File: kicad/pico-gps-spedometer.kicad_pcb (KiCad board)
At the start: 2 copper layers, 88.1 x 75.5 mm, 28 parts, among them J1 Akkumulátor be, J2 TP4056-18650-Charger, J3 uBlox NEO GPS (6M/8M), Q1 PN2222A, Q2 BC212, U1 RP2040-ZERO, U2 DS18B20, U3 LM7805_TO220, U4 TFT_320x240

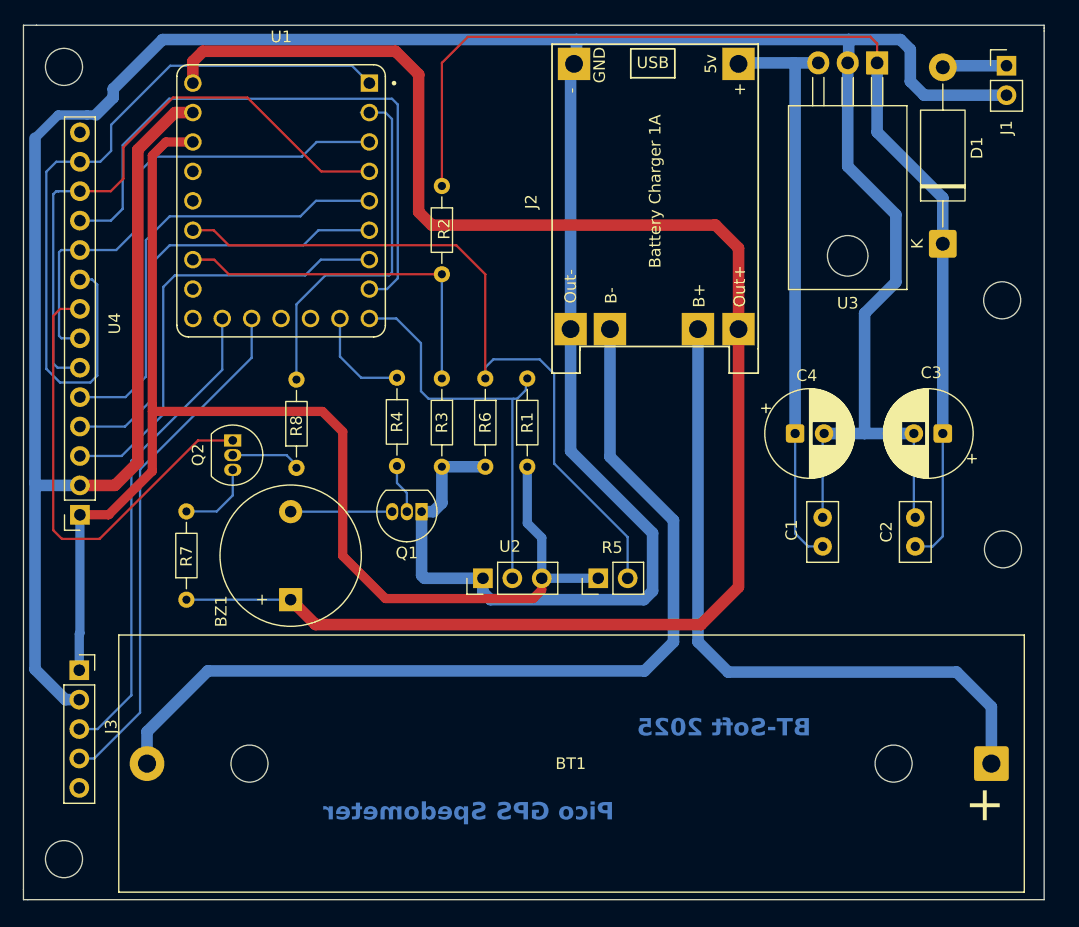
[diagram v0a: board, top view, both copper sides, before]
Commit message: Refactor code structure for improved readability and maintainability
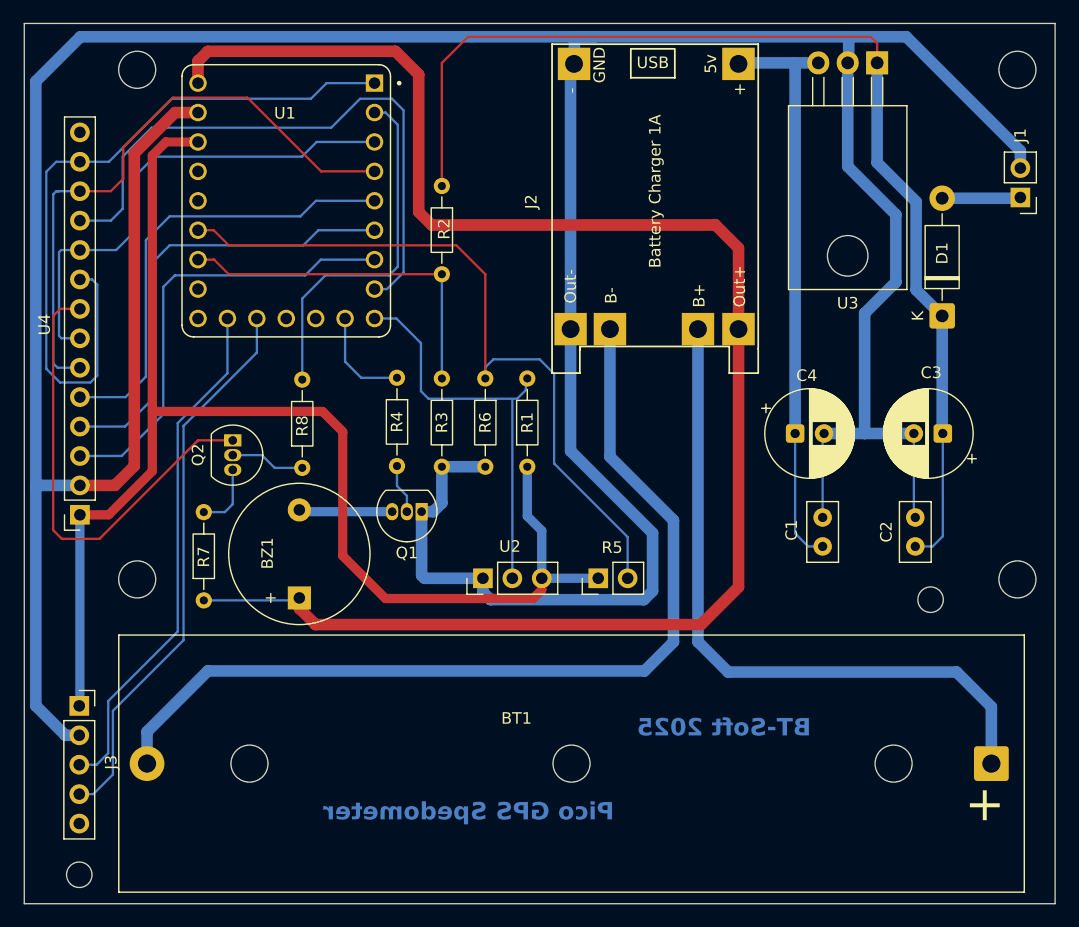
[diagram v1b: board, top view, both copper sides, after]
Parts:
- added ?: , , F.Cu at (99.5, 86.4)
- added REF**: MountingHole_2.2mm_M2, MountingHole:MountingHole_2.2mm_M2, F.Cu at (57.0, 96.0)
- added REF**: MountingHole_2.2mm_M2, MountingHole:MountingHole_2.2mm_M2, F.Cu at (130.5, 72.2)
- D1: footprint Diode_THT:D_DO-15_P15.24mm_Horizontal -> Diode_THT:D_DO-41_SOD81_P10.16mm_Horizontal
- moved REF** 25.0 mm to (62.0, 70.5)
- moved REF** 19.9 mm to (138.0, 26.5)
- moved J1 11.4 mm to (138.2, 37.5), turned to 180 degrees
- moved REF** 6.32 mm to (62.0, 26.5)
- moved D1 6.23 mm to (131.5, 47.8)
- moved J3 3.08 mm to (57.0, 81.4)
- moved REF** 2.88 mm to (138.0, 70.5)
- moved R7 1.50 mm to (67.8, 72.3)
- moved BZ1 0.76 mm to (76.0, 72.1)
- moved R8 0.50 mm to (76.2, 60.9)
- moved U1 0.45 mm to (74.9, 37.8)
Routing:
- net GND: track 332.4 -> 343.4 mm
- net GPS_TXD: track 41.5 -> 44.8 mm
- net GPS_RXD: track 44.9 -> 48.1 mm
- net +3V3: track 115.9 -> 118.9 mm
- net /MISO: track 65.3 -> 63.2 mm
- net +5VBATT: track 142.8 -> 141.5 mm
- net Net-(D1-A): track 5.55 -> 6.78 mm
- net Net-(Q2-E): track 6.78 -> 5.75 mm
- net Net-(U1-GP1): track 31.8 -> 31.1 mm
- net /T_CS: track 53.1 -> 52.5 mm
- net Net-(Q2-B): track 5.85 -> 6.46 mm
- net Net-(BZ1--): track 8.73 -> 8.15 mm
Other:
- board size 88.1 x 75.5 mm -> 89 x 76 mm
